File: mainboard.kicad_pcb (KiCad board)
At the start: 2 copper layers, 25 parts, among them J1 105017-1001, J2 XT60-M, Q1 AOD4184A, Q2 AOD4184A, U1 ESP32-WROOM-32E_(16MB), U2 CH340E, U3 AMS1117-3.3, U4 PAM8403DR

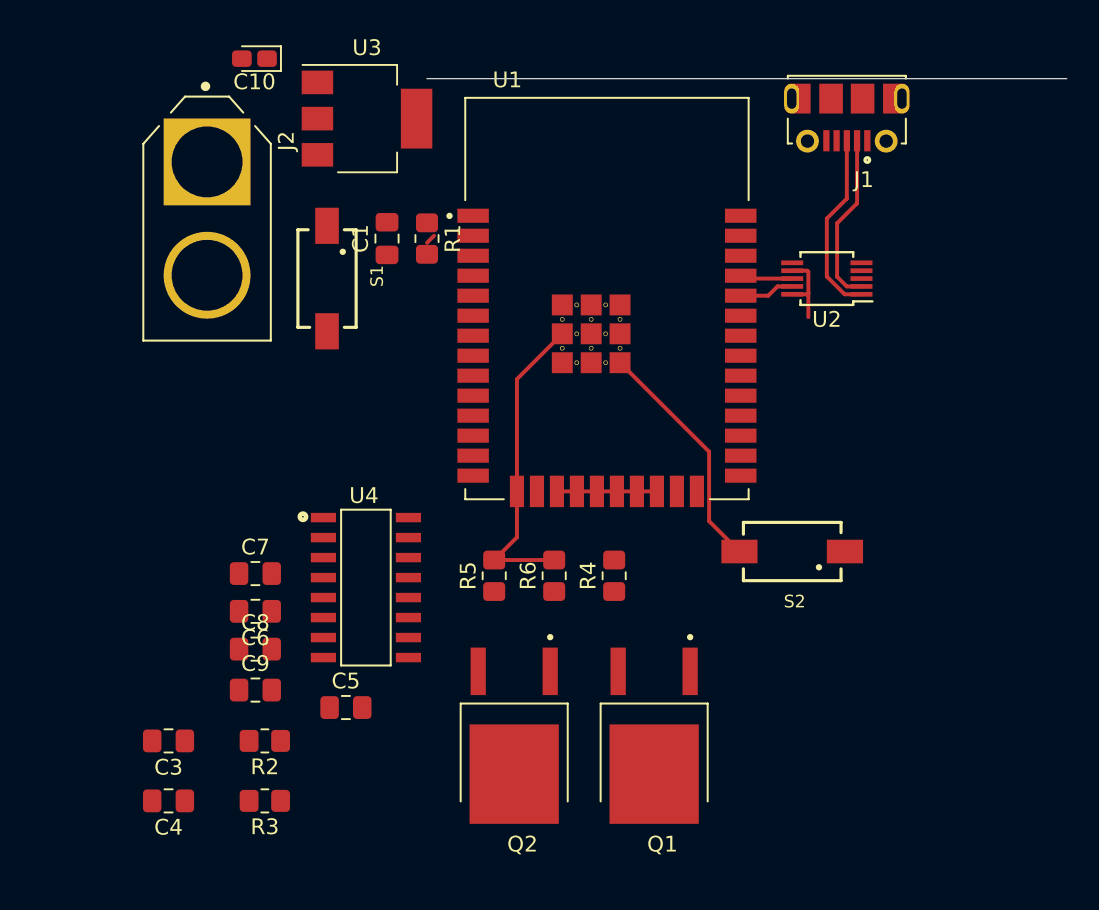
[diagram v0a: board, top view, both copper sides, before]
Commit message: sorry stef
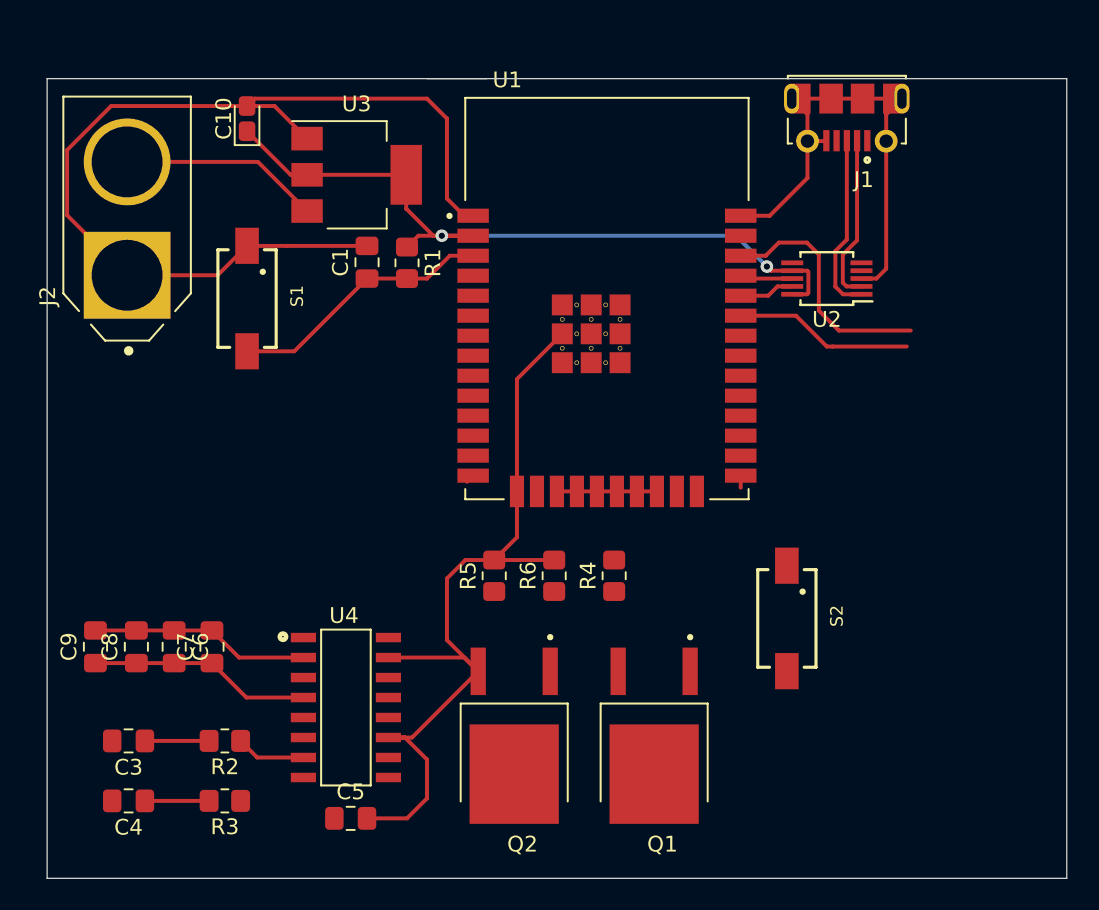
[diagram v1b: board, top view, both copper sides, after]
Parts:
- moved C9 10.5 mm to (42.4, 122.5), turned to 90 degrees
- moved U4 7.73 mm to (58.4, 126.3)
- moved C8 7.56 mm to (45.0, 122.5), turned to 90 degrees
- moved C5 7.05 mm to (58.7, 133.3)
- moved C6 5.63 mm to (47.4, 122.5), turned to 270 degrees
- moved C7 5.41 mm to (49.8, 122.5), turned to 90 degrees
- moved S1 5.24 mm to (52.1, 100.3)
- moved J2 5.08 mm to (44.5, 95.2), turned to 90 degrees
- moved S2 4.26 mm to (86.4, 120.7), turned to 270 degrees
- moved C10 3.84 mm to (52.1, 88.9), turned to 90 degrees
- moved U3 3.63 mm to (59.0, 92.5)
- moved C3 2.54 mm to (44.5, 128.4)
- moved C4 2.54 mm to (44.5, 132.2)
- moved R2 2.54 mm to (50.7, 128.4)
- moved R3 2.54 mm to (50.7, 132.2)
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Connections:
- net mute renamed Net-(U4-Pad5)
- U1 pad 14: Net-(U1-Pad14) -> SHND
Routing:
- net GND: track 35.1 -> 165.5 mm
- net 3V3: track 5.62 -> 49.5 mm, vias 0 -> 2
- net Net-(C1-Pad1): track 0.00 -> 16.9 mm
- net Net-(U1-Pad36): track 0.00 -> 15.5 mm
- net 5V: track 0.00 -> 14.1 mm
- net Net-(J2-Pad2): track 0.00 -> 12.7 mm
- net Net-(U1-Pad33): track 0.00 -> 11.4 mm
- net Net-(R2-Pad1): track 0.00 -> 4.43 mm
- net Net-(C4-Pad1): track 0.00 -> 4.08 mm
- net Net-(C3-Pad1): track 0.00 -> 4.08 mm
- net Net-(S2-Pad1): track 0.00 -> 0.77 mm
- net SHND: track 0.00 -> 0.55 mm
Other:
- board outline added: 64.8 x 50.8 mm
- board text added: "Ruimte voor connectors"
